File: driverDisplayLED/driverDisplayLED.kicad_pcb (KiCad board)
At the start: 2 copper layers, 36 parts, among them J1 Conn_01x12_Male, J2 Conn_01x12_Male, J3 Conn_01x12_Male, J4 Conn_02x08_Counter_Clockwise, J5 Conn_01x12_Male, J6 Conn_01x12_Male, J7 Conn_01x12_Male, J8 Conn_01x12_Male, J9 Conn_01x12_Male, Q1 FDS4953-FDS4953, Q2 FDS4953-FDS4953, Q3 FDS4953-FDS4953, Q4 FDS4953-FDS4953, U1 74HC245, U2 74HC595, U3 74HC595, U4 74HC245, U5 74HC138D, U6 74HC04, U7 74HC595, U8 74HC595

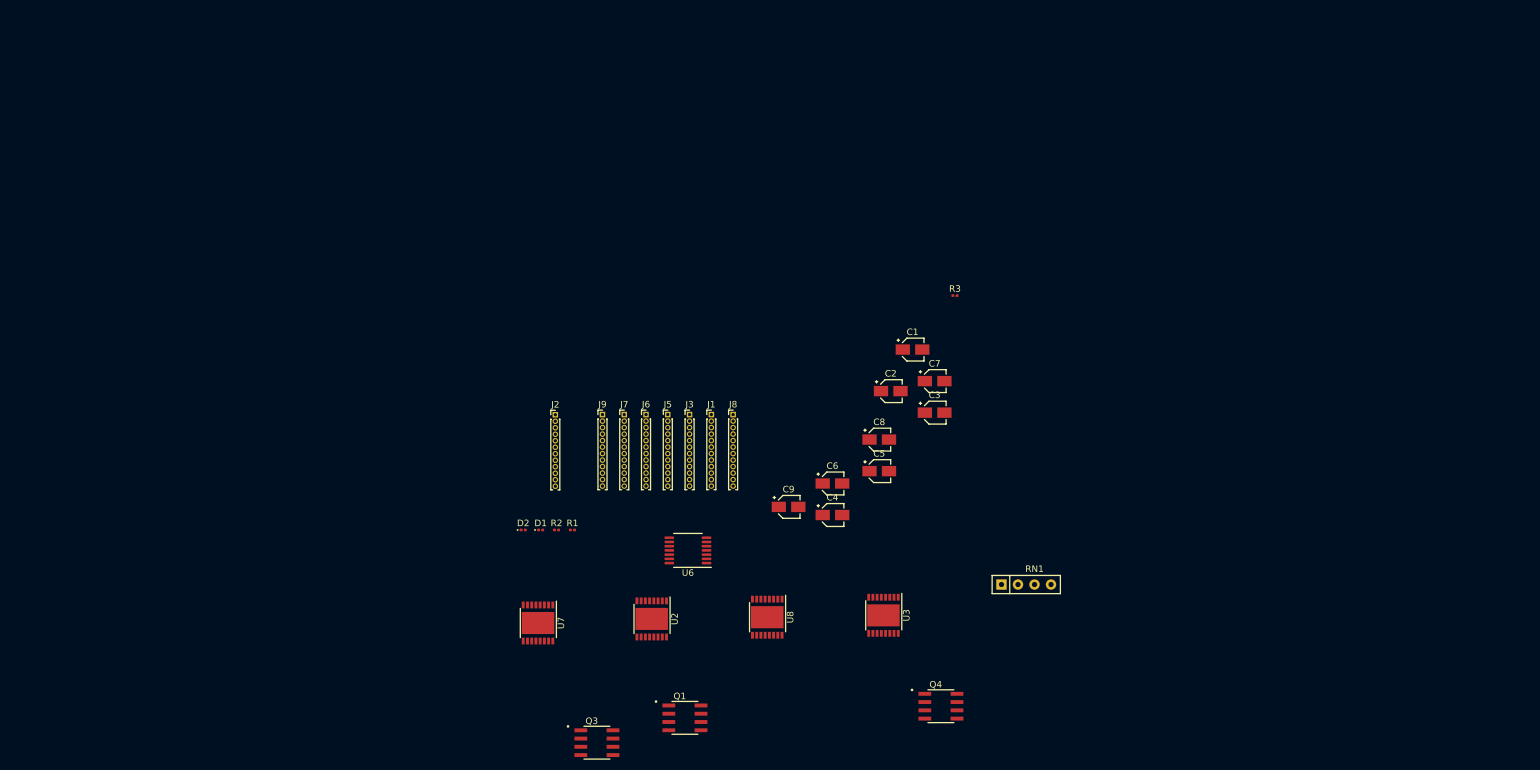
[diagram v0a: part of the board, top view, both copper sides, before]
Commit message: agrego borde PCB de muestra, y sus cotas
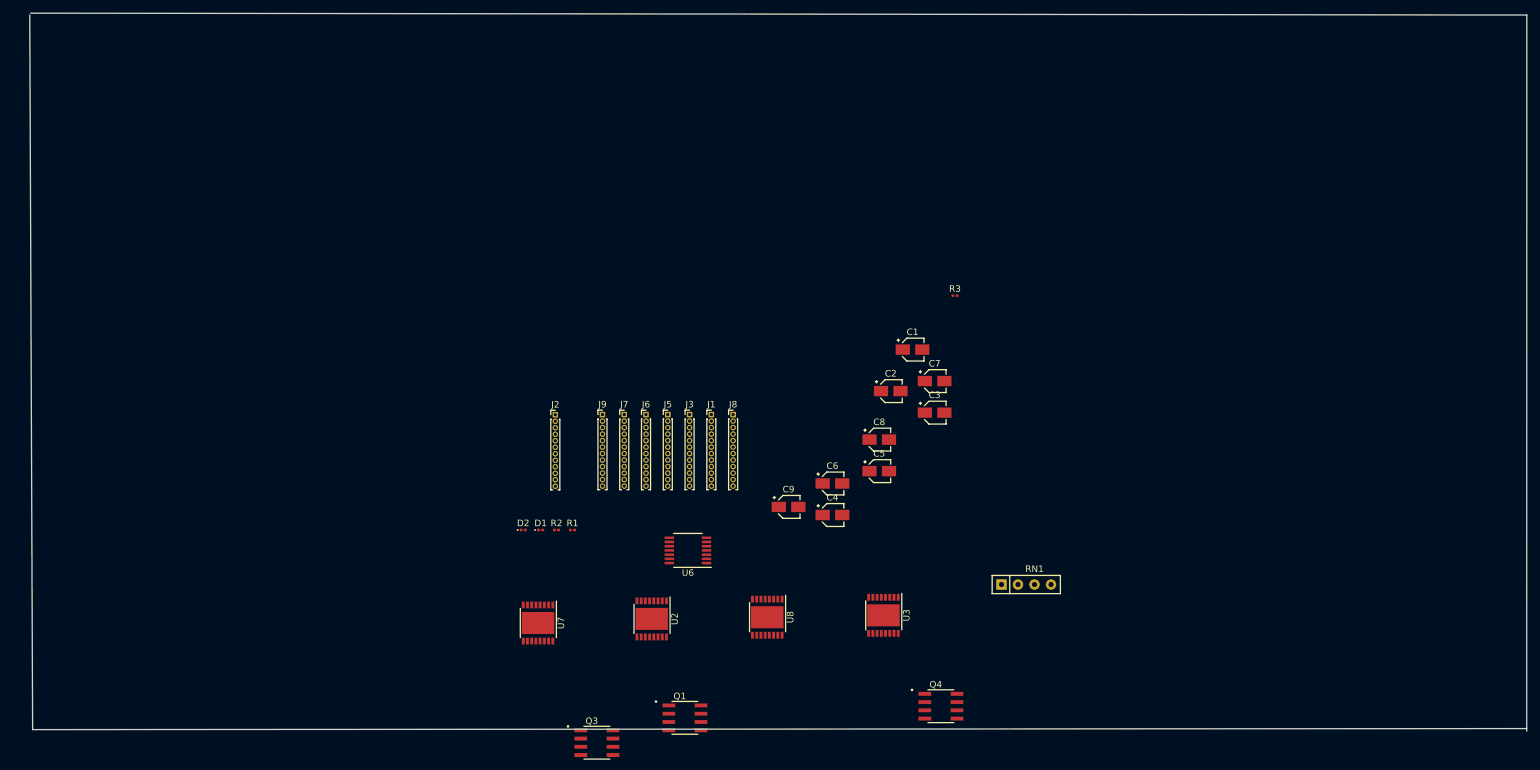
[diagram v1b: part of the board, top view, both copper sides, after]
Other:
- board outline added: 230.3 x 110.5 mm
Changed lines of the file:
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@@
   (general
     (thickness 1.6)
-    (drawings 0)
+    (drawings 6)
     (tracks 0)
     (zones 0)
@@
     )
   )
+  (dimension 230.290115 (width 0.15) (layer Dwgs.User)
+    (gr_text "230,290 mm" (at 145.108446 26.604694 359.9427764) (layer Dwgs.User)
+      (effects (font (size 1 1) (thickness 0.15)))
+    )
+    (feature1 (pts (xy 260.25 30.17) (xy 260.252733 27.433273)))
+    (feature2 (pts (xy 29.96 29.94) (xy 29.962733 27.203273)))
+    (crossbar (pts (xy 29.962148 27.789693) (xy 260.252148 28.019693)))
+    (arrow1a (pts (xy 260.252148 28.019693) (xy 259.125059 28.604988)))
+    (arrow1b (pts (xy 260.252148 28.019693) (xy 259.12623 27.432147)))
+    (arrow2a (pts (xy 29.962148 27.789693) (xy 31.088066 28.377239)))
+    (arrow2b (pts (xy 29.962148 27.789693) (xy 31.089237 27.204398)))
+  )
+  (dimension 109.920022 (width 0.15) (layer Dwgs.User)
+    (gr_text "109,920 mm" (at 263.344999 85.118045 270.0364875) (layer Dwgs.User)
+      (effects (font (size 1 1) (thickness 0.15)))
+    )
+    (feature1 (pts (xy 260.31 140.08) (xy 262.666419 140.078499)))
+    (feature2 (pts (xy 260.24 30.16) (xy 262.596419 30.158499)))
+    (crossbar (pts (xy 262.009999 30.158873) (xy 262.079999 140.078873)))
+    (arrow1a (pts (xy 262.079999 140.078873) (xy 261.492861 138.952743)))
+    (arrow1b (pts (xy 262.079999 140.078873) (xy 262.665702 138.951996)))
+    (arrow2a (pts (xy 262.009999 30.158873) (xy 261.424296 31.28575)))
+    (arrow2b (pts (xy 262.009999 30.158873) (xy 262.597137 31.285003)))
+  )
+  (gr_line (start 30.43 140.04) (end 29.99 30.09) (layer Edge.Cuts) (width 0.05))
+  (gr_line (start 260.28 139.88) (end 30.43 140.04) (layer Edge.Cuts) (width 0.05))
+  (gr_line (start 260.3 30.11) (end 260.28 140.28) (layer Edge.Cuts) (width 0.05))
+  (gr_line (start 30.14 29.82) (end 260.3 30.11) (layer Edge.Cuts) (width 0.05))
 )

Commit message: agrego modulo myLedMatrix. Probar instanciar debido al path local
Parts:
- moved C1 475.0 mm to (598.1, 278.6)
- moved C2 475.0 mm to (594.7, 285.0)
- moved C3 475.0 mm to (601.5, 288.3)
- moved C5 475.0 mm to (592.9, 297.3)
- moved C7 475.0 mm to (601.5, 283.4)
- moved C8 475.0 mm to (592.9, 292.4)
- moved D1 475.0 mm to (540.9, 306.3)
- moved J4 475.0 mm to (490.5, 357.4)
- moved J6 475.0 mm to (557.1, 288.6)
- moved J7 475.0 mm to (553.7, 288.6)
- moved J8 475.0 mm to (570.5, 288.6)
- moved R3 475.0 mm to (604.6, 270.3)
- moved U2 475.0 mm to (557.9, 320.0)
- moved U3 475.0 mm to (593.6, 319.4)
- moved U4 475.0 mm to (518.4, 367.6)
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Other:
- board size 230.3 x 110.5 mm -> 906 x 496.6 mm

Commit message: place components into PCB
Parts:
- added C10: C, Capacitor_SMD:CP_Elec_3x5.3, F.Cu at (157.4, 187.5)
- added C11: C, Capacitor_SMD:CP_Elec_3x5.3, F.Cu at (157.4, 182.6)
- added C12: C, Capacitor_SMD:CP_Elec_3x5.3, F.Cu at (157.4, 177.8)
- added C13: C, Capacitor_SMD:CP_Elec_3x5.3, F.Cu at (140.3, 196.1)
- added J10: Conn_01x12_Male, Connector_PinHeader_1.00mm:PinHeader_1x12_P1.00mm_Vertical, F.Cu at (98.0, 20.0)
- added J11: Conn_01x12_Male, Connector_PinHeader_1.00mm:PinHeader_1x12_P1.00mm_Vertical, F.Cu at (98.0, 24.0)
- added J12: Conn_01x12_Male, Connector_PinHeader_1.00mm:PinHeader_1x12_P1.00mm_Vertical, F.Cu at (98.0, 32.0)
- added J13: Conn_01x12_Male, Connector_PinHeader_1.00mm:PinHeader_1x12_P1.00mm_Vertical, F.Cu at (98.0, 37.0)
- added J14: Conn_01x12_Male, Connector_PinHeader_1.00mm:PinHeader_1x12_P1.00mm_Vertical, F.Cu at (116.0, 20.0)
- added J15: Conn_01x12_Male, Connector_PinHeader_1.00mm:PinHeader_1x12_P1.00mm_Vertical, F.Cu at (116.0, 24.0)
- added J16: Conn_01x12_Male, Connector_PinHeader_1.00mm:PinHeader_1x12_P1.00mm_Vertical, F.Cu at (116.0, 32.0)
- added J17: Conn_01x12_Male, Connector_PinHeader_1.00mm:PinHeader_1x12_P1.00mm_Vertical, F.Cu at (116.0, 37.0)
- added J18: Conn_02x08_Counter_Clockwise, Connector_PinHeader_2.54mm:PinHeader_2x08_P2.54mm_Vertical, F.Cu at (337.5, 105.0)
- added Q5: FDS4953, FDS4953:SOIC127P600X175-8N, F.Cu at (160.6, 117.5)
- added Q6: FDS4953, FDS4953:SOIC127P600X175-8N, F.Cu at (275.0, 117.5)
- added Q7: FDS4953, FDS4953:SOIC127P600X175-8N, F.Cu at (167.5, 117.5)
- added Q8: FDS4953, FDS4953:SOIC127P600X175-8N, F.Cu at (282.5, 117.5)
- added RN2: R_Network04, Resistor_THT:R_Array_SIP4, F.Cu at (108.9, 196.6)
- added RN3: R_Network04, Resistor_THT:R_Array_SIP4, F.Cu at (129.5, 178.2)
- added RN4: R_Network04, Resistor_THT:R_Array_SIP4, F.Cu at (134.9, 144.2)
- added RN5: R_Network04, Resistor_THT:R_Array_SIP4, F.Cu at (108.9, 192.3)
- added U10: 74HC595, Package_SO:HTSSOP-16-1EP_4.4x5mm_P0.65mm_EP3.4x5mm, F.Cu at (220.0, 75.0)
- added U11: 74HC595, Package_SO:HTSSOP-16-1EP_4.4x5mm_P0.65mm_EP3.4x5mm, F.Cu at (260.0, 75.0)
- added U12: 74HC595, Package_SO:HTSSOP-16-1EP_4.4x5mm_P0.65mm_EP3.4x5mm, F.Cu at (295.0, 75.0)
- added U13: 74HC595, Package_SO:HTSSOP-16-1EP_4.4x5mm_P0.65mm_EP3.4x5mm, F.Cu at (335.0, 75.0)
- added U9: 74HC138D, Package_SO:TSSOP-16_4.4x5mm_P0.65mm, F.Cu at (190.0, 115.0)
- Q1, Q2, Q3, Q4: value FDS4953-FDS4953 -> FDS4953
- moved J1 568.5 mm to (66.0, 20.0), turned to 270 degrees
- moved J3 560.0 mm to (66.0, 32.0), turned to 270 degrees
- moved J5 554.7 mm to (66.0, 37.0), turned to 270 degrees
- moved J8 551.7 mm to (82.0, 32.0), turned to 270 degrees
- moved U2 546.0 mm to (70.0, 75.0), turned to 90 degrees
- moved J6 545.7 mm to (82.0, 20.0), turned to 270 degrees
- moved J2 545.6 mm to (66.0, 24.0), turned to 270 degrees
- moved U3 541.9 mm to (110.0, 75.0), turned to 90 degrees
- moved J7 540.8 mm to (82.0, 24.0), turned to 270 degrees
- moved J9 531.6 mm to (82.0, 37.0), turned to 270 degrees
- moved U6 495.1 mm to (127.5, 75.0), turned to 90 degrees
- moved U5 489.8 mm to (120.0, 117.5)
- moved U4 486.6 mm to (102.5, 115.0)
- moved Q1 484.7 mm to (130.0, 117.5), turned to 90 degrees
- moved J4 484.1 mm to (77.5, 105.0)
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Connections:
- net /B4-E3 renamed Net-(U4-Pad14)
- net /B5-E2 renamed Net-(U4-Pad13)
- net Net-(U1-Pad6) renamed LT
- net Net-(U1-Pad9) renamed SRCLK-2
- J1 pad 1: GND -> /R8
- J1 pad 10: /R6 -> /H3
- J1 pad 11: /R7 -> /H2
- J1 pad 12: /R8 -> /H1
- J1 pad 2: GND -> /R7
- J1 pad 3: GND -> /R6
- J1 pad 4: GND -> /R5
- J1 pad 5: /R1 -> /R4
- J1 pad 6: /R2 -> /R3
- J1 pad 7: /R3 -> /R2
- J1 pad 8: /R4 -> /R1
- J1 pad 9: /R5 -> /H4
- J2 pad 1: /H8 -> /G8
- J2 pad 10: /G6 -> /H6
- J2 pad 11: /G7 -> /H7
- J2 pad 12: /G8 -> /H8
- J2 pad 2: /H7 -> /G7
- J2 pad 3: /H6 -> /G6
- J2 pad 4: /H5 -> /G5
- J2 pad 5: /G1 -> /G4
- J2 pad 6: /G2 -> /G3
- J2 pad 7: /G3 -> /G2
- J2 pad 8: /G4 -> /G1
- J2 pad 9: /G5 -> /H5
- J3 pad 1: /H8 -> /R8
- J3 pad 10: /G6 -> /H3
- J3 pad 11: /G7 -> /H2
- J3 pad 12: /G8 -> /H1
- J3 pad 2: /H7 -> /R7
- J3 pad 3: /H6 -> /R6
- J3 pad 4: /H5 -> /R5
- J3 pad 5: /G1 -> /R4
- J3 pad 6: /G2 -> /R3
- J3 pad 7: /G3 -> /R2
- J3 pad 8: /G4 -> /R1
- J3 pad 9: /G5 -> /H4
- J5 pad 1: GND -> /G8
- J5 pad 10: /R6 -> /H6
- J5 pad 11: /R7 -> /H7
- J5 pad 12: /R8 -> /H8
- J5 pad 2: GND -> /G7
- J5 pad 3: GND -> /G6
- J5 pad 4: GND -> /G5
- J5 pad 5: /R1 -> /G4
- J5 pad 6: /R2 -> /G3
- J5 pad 7: /R3 -> /G2
- J5 pad 8: /R4 -> /G1
- J5 pad 9: /R5 -> /H5
- J6 pad 1: /H8 -> /R8
- J6 pad 10: /G6 -> /H3
- J6 pad 11: /G7 -> /H2
- J6 pad 12: /G8 -> /H1
- J6 pad 2: /H7 -> /R7
- J6 pad 3: /H6 -> /R6
- J6 pad 4: /H5 -> /R5
- J6 pad 5: /G1 -> /R4
- J6 pad 6: /G2 -> /R3
- J6 pad 7: /G3 -> /R2
- J6 pad 8: /G4 -> /R1
- J6 pad 9: /G5 -> /H4
- J7 pad 1: /H8 -> /G8
- J7 pad 10: /G6 -> /H6
- J7 pad 11: /G7 -> /H7
- J7 pad 12: /G8 -> /H8
- J7 pad 2: /H7 -> /G7
- J7 pad 3: /H6 -> /G6
- J7 pad 4: /H5 -> /G5
- J7 pad 5: /G1 -> /G4
- J7 pad 6: /G2 -> /G3
- J7 pad 7: /G3 -> /G2
- J7 pad 8: /G4 -> /G1
- J7 pad 9: /G5 -> /H5
- J8 pad 1: GND -> /R8
- J8 pad 10: /R6 -> /H3
- J8 pad 11: /R7 -> /H2
- J8 pad 12: /R8 -> /H1
- J8 pad 2: GND -> /R7
- J8 pad 3: GND -> /R6
- J8 pad 4: GND -> /R5
- J8 pad 5: /R1 -> /R4
- J8 pad 6: /R2 -> /R3
- J8 pad 7: /R3 -> /R2
- J8 pad 8: /R4 -> /R1
- J8 pad 9: /R5 -> /H4
- J9 pad 1: GND -> /G8
- J9 pad 10: /R6 -> /H6
- J9 pad 11: /R7 -> /H7
- J9 pad 12: /R8 -> /H8
- J9 pad 2: GND -> /G7
- J9 pad 3: GND -> /G6
- J9 pad 4: GND -> /G5
- J9 pad 5: /R1 -> /G4
- J9 pad 6: /R2 -> /G3
- J9 pad 7: /R3 -> /G2
- J9 pad 8: /R4 -> /G1
- J9 pad 9: /R5 -> /H5
- Q1 pad 1: /1 -> VCC
- Q1 pad 2: /2 -> /Y1-G1
- Q1 pad 3: /3 -> VCC
- Q1 pad 4: /4 -> /Y0-G2
- Q1 pad 5: /5 -> /D2-H1
- Q1 pad 6: /5 -> /D2-H1
- Q1 pad 7: /7 -> /D1-H2
- Q1 pad 8: /7 -> /D1-H2
- Q2 pad 1: /1 -> VCC
- Q2 pad 2: /2 -> /Y1-G1
- Q2 pad 3: /3 -> VCC
- Q2 pad 4: /4 -> /Y0-G2
- Q2 pad 5: /5 -> /D2-H1
- Q2 pad 6: /5 -> /D2-H1
- Q2 pad 7: /7 -> /D1-H2
- Q2 pad 8: /7 -> /D1-H2
- Q3 pad 1: /1 -> VCC
- Q3 pad 2: /2 -> /Y3-G1
- Q3 pad 3: /3 -> VCC
- Q3 pad 4: /4 -> /Y2-G2
- Q3 pad 5: /5 -> /D2-H3
- Q3 pad 6: /5 -> /D2-H3
- Q3 pad 7: /7 -> /D1-H4
- Q3 pad 8: /7 -> /D1-H4
- Q4 pad 1: /1 -> VCC
- Q4 pad 2: /2 -> /Y3-G1
- Q4 pad 3: /3 -> VCC
- Q4 pad 4: /4 -> /Y2-G2
- Q4 pad 5: /5 -> /D2-H3
- Q4 pad 6: /5 -> /D2-H3
- Q4 pad 7: /7 -> /D1-H4
- Q4 pad 8: /7 -> /D1-H4
- R2 pad 1: Net-(R2-Pad1) -> Net-(C6-Pad1)
- RN1 pad 1: Net-(RN1-Pad1) -> GND
- RN1 pad 2: Net-(RN1-Pad2) -> /D2-H1
- RN1 pad 3: Net-(RN1-Pad3) -> /D1-H2
- RN1 pad 4: Net-(RN1-Pad4) -> /D2-H3
- U1 pad 1: Net-(U1-Pad1) -> GND
- U1 pad 19: Net-(U1-Pad19) -> GND
- U2 pad 1: Net-(U2-Pad1) -> /R7
- U2 pad 15: Net-(U2-Pad15) -> /R8
- U2 pad 2: Net-(U2-Pad2) -> /R6
- U2 pad 3: Net-(U2-Pad3) -> /R5
- U2 pad 4: Net-(U2-Pad4) -> /R4
- U2 pad 5: Net-(U2-Pad5) -> /R3
- U2 pad 6: Net-(U2-Pad6) -> /R2
- U2 pad 7: Net-(U2-Pad7) -> /R1
- U3 pad 9: /QH-SER -> Net-(U3-Pad9)
- U5 pad 12: /4 -> Net-(U5-Pad12)
- U5 pad 13: /2 -> Net-(U5-Pad13)
- U5 pad 14: /4 -> Net-(U5-Pad14)
- U5 pad 15: /2 -> Net-(U5-Pad15)
- U5 pad 4: Net-(U5-Pad4) -> /E1
- U6 pad 1: Net-(R2-Pad1) -> Net-(C6-Pad1)
- U6 pad 10: Net-(U6-Pad10) -> (no net)
- U6 pad 11: VCC -> (no net)
- U6 pad 12: Net-(U6-Pad12) -> (no net)
- U6 pad 13: VCC -> (no net)
- U6 pad 4: Net-(U6-Pad4) -> /E1
- U6 pad 5: Net-(U6-Pad4) -> /E1
- U6 pad 6: Net-(U6-Pad6) -> /E3
- U6 pad 8: Net-(U6-Pad8) -> (no net)
- U6 pad 9: VCC -> (no net)
- U7 pad 14: /A1-SER -> Net-(U3-Pad9)
- U7 pad 9: /QH-SER -> Net-(U7-Pad9)
- U8 pad 14: /A1-SER -> Net-(U7-Pad9)
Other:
- board outline removed
